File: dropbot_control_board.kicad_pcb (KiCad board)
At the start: 2 copper layers, 83.8 x 56.1 mm, 60 parts, among them J2 COMM_BUS, P3 POWER, P4 VOUT, P5 LIGHT, P6 MAGNET, P7 CONN_01X05, P8 CONN_01X03, Q1 IRF644PBF, Q2 TIP120, Q3 2N7002, Q4 2N7002, Q5 Q_NMOS_GDS, Q6 Q_NMOS_GDS, U1 Teensy_3.1, U2 MAX1771, U3 MCP41050, U4 HV7802, U5 AQW216, U6 NCP5304

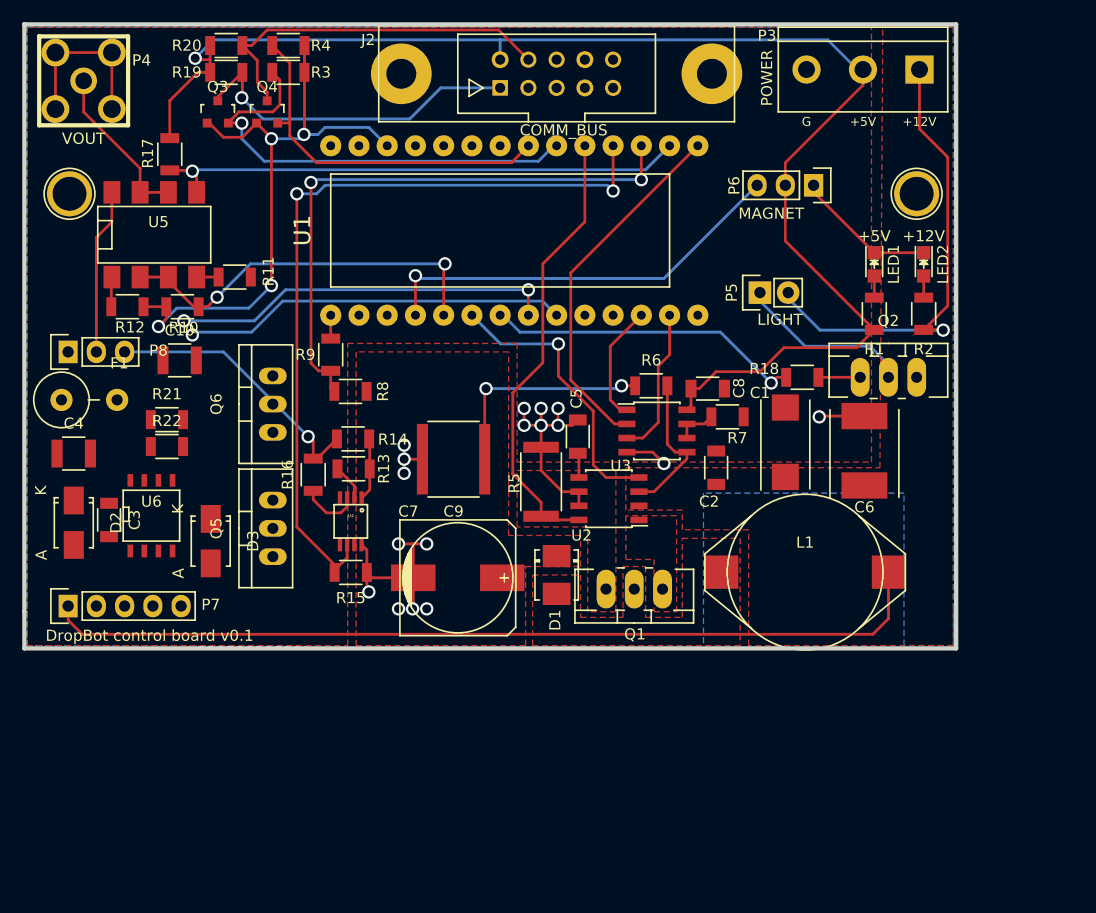
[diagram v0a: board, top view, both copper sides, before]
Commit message: Re-do layout
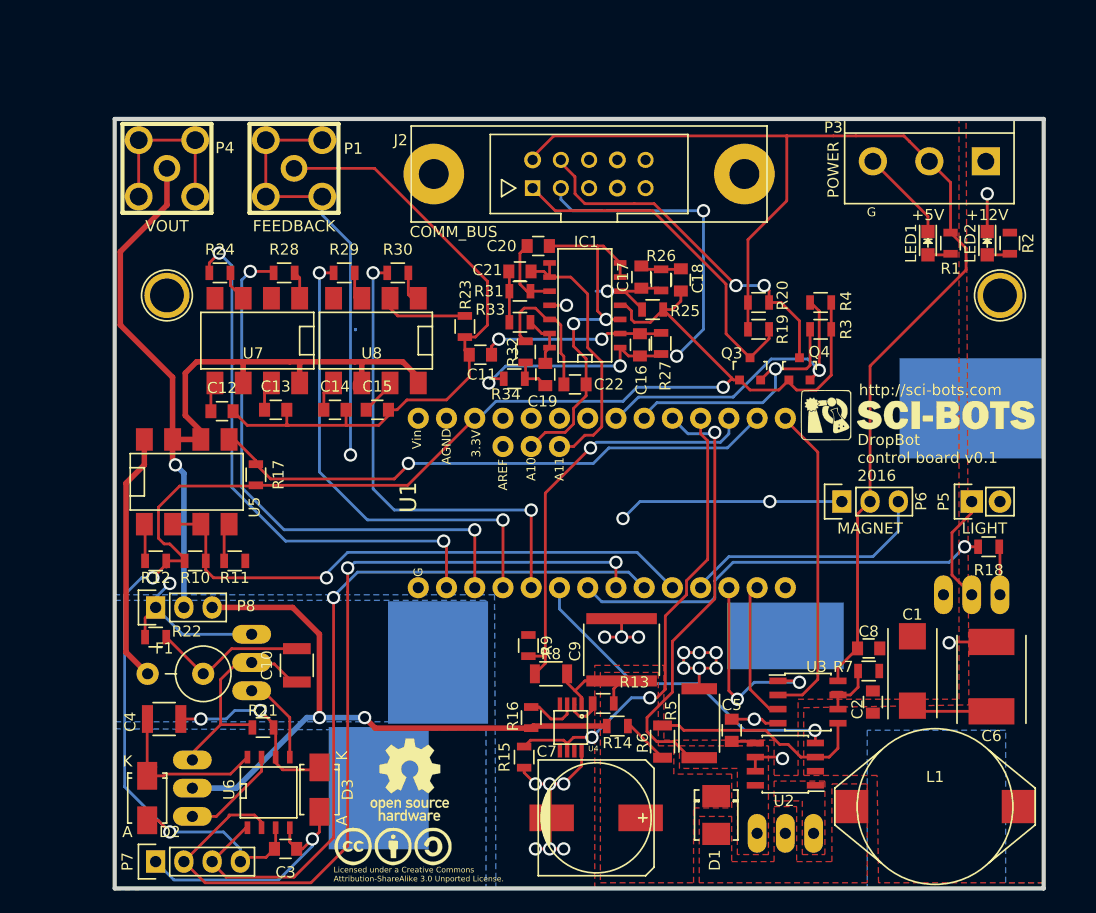
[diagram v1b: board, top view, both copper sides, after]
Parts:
- added C11: 1uF, Capacitors_SMD:C_0805, F.Cu at (57.3, 45.0)
- added C12: 1pF, Capacitors_SMD:C_0805, F.Cu at (34.0, 50.0)
- added C13: 10pF, Capacitors_SMD:C_0805, F.Cu at (38.9, 49.9)
- added C14: 100pF, Capacitors_SMD:C_0805, F.Cu at (44.2, 49.9)
- added C15: 1nF, Capacitors_SMD:C_0805, F.Cu at (48.0, 49.9)
- added C16: 0.1uF, Capacitors_SMD:C_0805, F.Cu at (71.6, 44.1)
- added C17: 0.1uF, Capacitors_SMD:C_0805, F.Cu at (71.8, 38.0)
- added C18: 0.1uF, Capacitors_SMD:C_0805, F.Cu at (75.3, 38.2)
- added C19: 4.7nF, Capacitors_SMD:C_0805, F.Cu at (63.1, 46.7)
- added C20: 1nF, Capacitors_SMD:C_0805, F.Cu at (62.5, 35.2)
- added C21: 0.15uF, Capacitors_SMD:C_0805, F.Cu at (60.8, 37.5)
- added C22: 1nF, Capacitors_SMD:C_0805, F.Cu at (65.8, 47.6)
- added G***: LOGO, LOGO, F.Cu at (49.4, 89.2)
- added G***: LOGO, LOGO, F.Cu at (50.9, 83.2)
- added G***: LOGO, LOGO, F.Cu at (96.6, 50.4)
- added IC1: MCP6024, SMD_Packages:SOIC-14_N, F.Cu at (66.5, 40.5)
- added P1: FEEDBACK, footprints:JACK_SMA, F.Cu at (40.5, 28.2)
- added R23: 1Meg, Resistors_SMD:R_0805, F.Cu at (55.9, 42.4)
- added R24: 200, Resistors_SMD:R_0805, F.Cu at (33.8, 37.6)
- added R25: 10k, Resistors_SMD:R_0805, F.Cu at (72.8, 40.9)
- added R26: 2.2k, Resistors_SMD:R_0805, F.Cu at (73.5, 38.2)
- added R27: 1Meg, Resistors_SMD:R_0805, F.Cu at (73.5, 43.9)
- added R28: 200, Resistors_SMD:R_0805, F.Cu at (39.6, 37.6)
- added R29: 200, Resistors_SMD:R_0805, F.Cu at (45.0, 37.6)
- added R30: 200, Resistors_SMD:R_0805, F.Cu at (49.8, 37.6)
- added R31: 1.91k, Resistors_SMD:R_0805, F.Cu at (60.8, 39.2)
- added R32: 16.9k, Resistors_SMD:R_0805, F.Cu at (61.3, 44.7)
- added R33: 806, Resistors_SMD:R_0805, F.Cu at (60.8, 42.0)
- added R34: 13.3k, Resistors_SMD:R_0805, F.Cu at (60.3, 47.1)
- added U7: AQW216, SMD_Packages:DIP-8_SMD, F.Cu at (37.2, 43.7)
- added U8: AQW216, SMD_Packages:DIP-8_SMD, F.Cu at (47.9, 43.7)
- C2, C3, C5, C8: footprint Capacitors_SMD:C_1206 -> Capacitors_SMD:C_0805
- P7: value CONN_01X05 -> CONN_01X04; footprint Pin_Headers:Pin_Header_Straight_1x05 -> Pin_Headers:Pin_Header_Straight_1x04
- Q1, Q2: footprint TO_SOT_Packages_THT:TO-220_Neutral123_Vertical_LargePads -> TO_SOT_Packages_THT:TO-220_Neutral123_Horizontal_LargePads; moved to B.Cu
- Q5, Q6: footprint TO_SOT_Packages_THT:TO-220_Neutral123_Vertical -> TO_SOT_Packages_THT:TO-220_Neutral123_Horizontal_LargePads; moved to B.Cu
- R1, R10, R11, R12, R13, R14, R15, R16, R17, R18, R19, R2, R20, R21, R22, R3, R4, R7, R9: footprint Resistors_SMD:R_1206 -> Resistors_SMD:R_0805
- U1: value Teensy_3.1 -> Teensy_3.2; footprint footprints:Teensy-3.1 -> footprints:Teensy-3.2
- moved Q3 53.2 mm to (81.5, 46.2)
- moved R19 53.2 mm to (82.3, 42.7)
- moved R20 53.2 mm to (82.3, 40.3)
- moved Q4 53.2 mm to (86.0, 46.2)
- moved R3 53.2 mm to (87.9, 42.7)
- moved R4 53.2 mm to (87.9, 40.3)
- moved R14 35.1 mm to (69.6, 78.4)
- moved C3 33.6 mm to (39.8, 89.4), turned to 180 degrees
- moved R6 32.0 mm to (73.7, 79.8), turned to 90 degrees
- moved R9 31.6 mm to (61.6, 71.1)
- moved R8 31.2 mm to (63.6, 73.7)
- moved R13 30.8 mm to (68.3, 76.3)
- moved R17 29.9 mm to (37.1, 55.8), turned to 90 degrees
- moved C5 29.8 mm to (79.9, 78.7)
- moved C10 29.4 mm to (40.8, 72.9), turned to 90 degrees
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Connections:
- C3 pad 2: +5V -> +3.3V
- D2 pad 2: +5V -> +3.3V
- F1 pad 2: VOUT -> HVAC
- P4 pad 1: Net-(P4-Pad1) -> VOUT
- P6 pad 3: D2/SERVO -> D9/SERVO
- P7 pad 1: +12V -> GND
- P7 pad 2: GND -> D6/DRIVER_HI
- P7 pad 3: D6/DRIVER_HI -> D7/DRIVER_LO
- P7 pad 4: D7/DRIVER_LO -> +3.3V
- R10 pad 2: D3/OUTPUT_SELECT -> D8/OUTPUT_SELECT
- R17 pad 1: +5V -> +3.3V
- U1 pad 0: Net-(U1-Pad0) -> D0
- U1 pad 1: Net-(U1-Pad1) -> D1
- U1 pad 2: D2/SERVO -> D2
- U1 pad 3: D3/OUTPUT_SELECT -> D3
- U1 pad 8: Net-(U1-Pad8) -> D8/OUTPUT_SELECT
- U1 pad 9: Net-(U1-Pad9) -> D9/SERVO
- U5 pad 2: D3/OUTPUT_SELECT -> D8/OUTPUT_SELECT
- U5 pad 3: D3/OUTPUT_SELECT -> D8/OUTPUT_SELECT
- U5 pad 6: Net-(P4-Pad1) -> VOUT
- U5 pad 7: Net-(P4-Pad1) -> VOUT
- U5 pad 8: VOUT -> HVAC
- U6 pad 3: +5V -> +3.3V
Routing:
- net GND: track 84.1 -> 210.8 mm, vias 17 -> 27
- net +12V: track 123.1 -> 7.32 mm, vias 1 -> 0
- net +3.3V: track 56.1 -> 143.3 mm, vias 4 -> 3
- net VOUT: track 15.0 -> 81.7 mm, vias 0 -> 1
- net CUR_SENSE: track 0.00 -> 58.7 mm
- net D8/OUTPUT_SELECT: track 0.00 -> 51.7 mm, vias 0 -> 1
- net D1: track 0.00 -> 49.9 mm, vias 0 -> 2
- net D0: track 0.00 -> 49.0 mm, vias 0 -> 2
- net D6/DRIVER_HI: track 34.4 -> 78.1 mm
- net D2: track 0.00 -> 43.6 mm, vias 0 -> 2
- net D3: track 0.00 -> 42.7 mm, vias 0 -> 2
- net D2/SERVO: track 37.9 -> 0.00 mm, vias 1 -> 0
- net D3/OUTPUT_SELECT: track 35.4 -> 0.00 mm, vias 2 -> 0
- net +0.6V: track 0.00 -> 34.3 mm, vias 0 -> 2
- net HV: track 25.0 -> 58.8 mm, vias 1 -> 2
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- added copper zone on B.Cu, net HV
- added copper zone on B.Cu, net Net-(C10-Pad1)
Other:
- board size 83.8 x 56.1 mm -> 83.6 x 69.2 mm
- net class PWR added: clearance 0.127, trace_width 0.5, via_dia 1.2, via_drill 0.8
- board text added: "DropBot control board v0.1 2016"
- board text added: "Licensed under a Creative Commons Attribution-ShareAlike 3.0 Unported License."
- board text added: "http://sci-bots.com"
- board text removed: "+12V"
- board text removed: "+5V"
- board text removed: "DropBot control board v0.1"
